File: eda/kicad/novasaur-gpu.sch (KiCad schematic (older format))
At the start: 24 parts, among them U1 74F86, U28 74F163, U29 74F163, U3 74F11, U30 74F541, U31 74F574, U32 74F574, U33 74F541, U34 74F574, U35 74F299, U36 74F574, U37 74F157

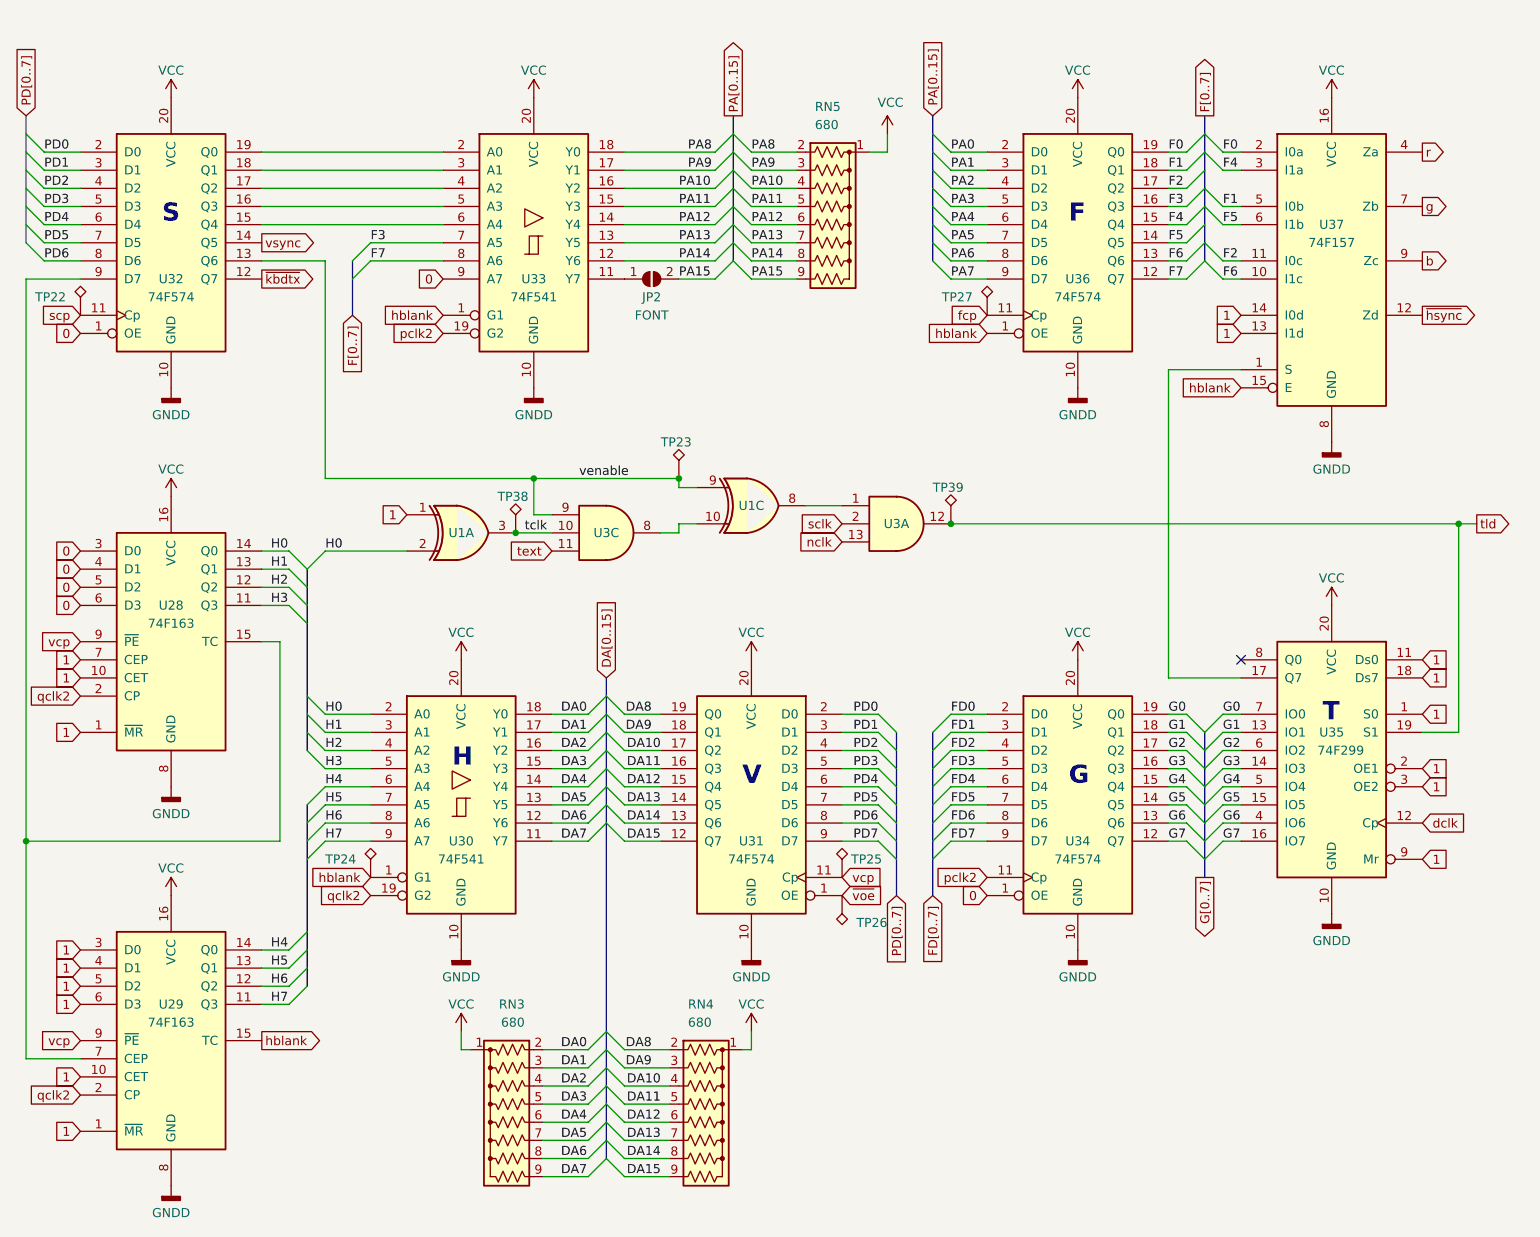
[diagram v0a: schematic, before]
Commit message: Rev. 10 with 5v PSU
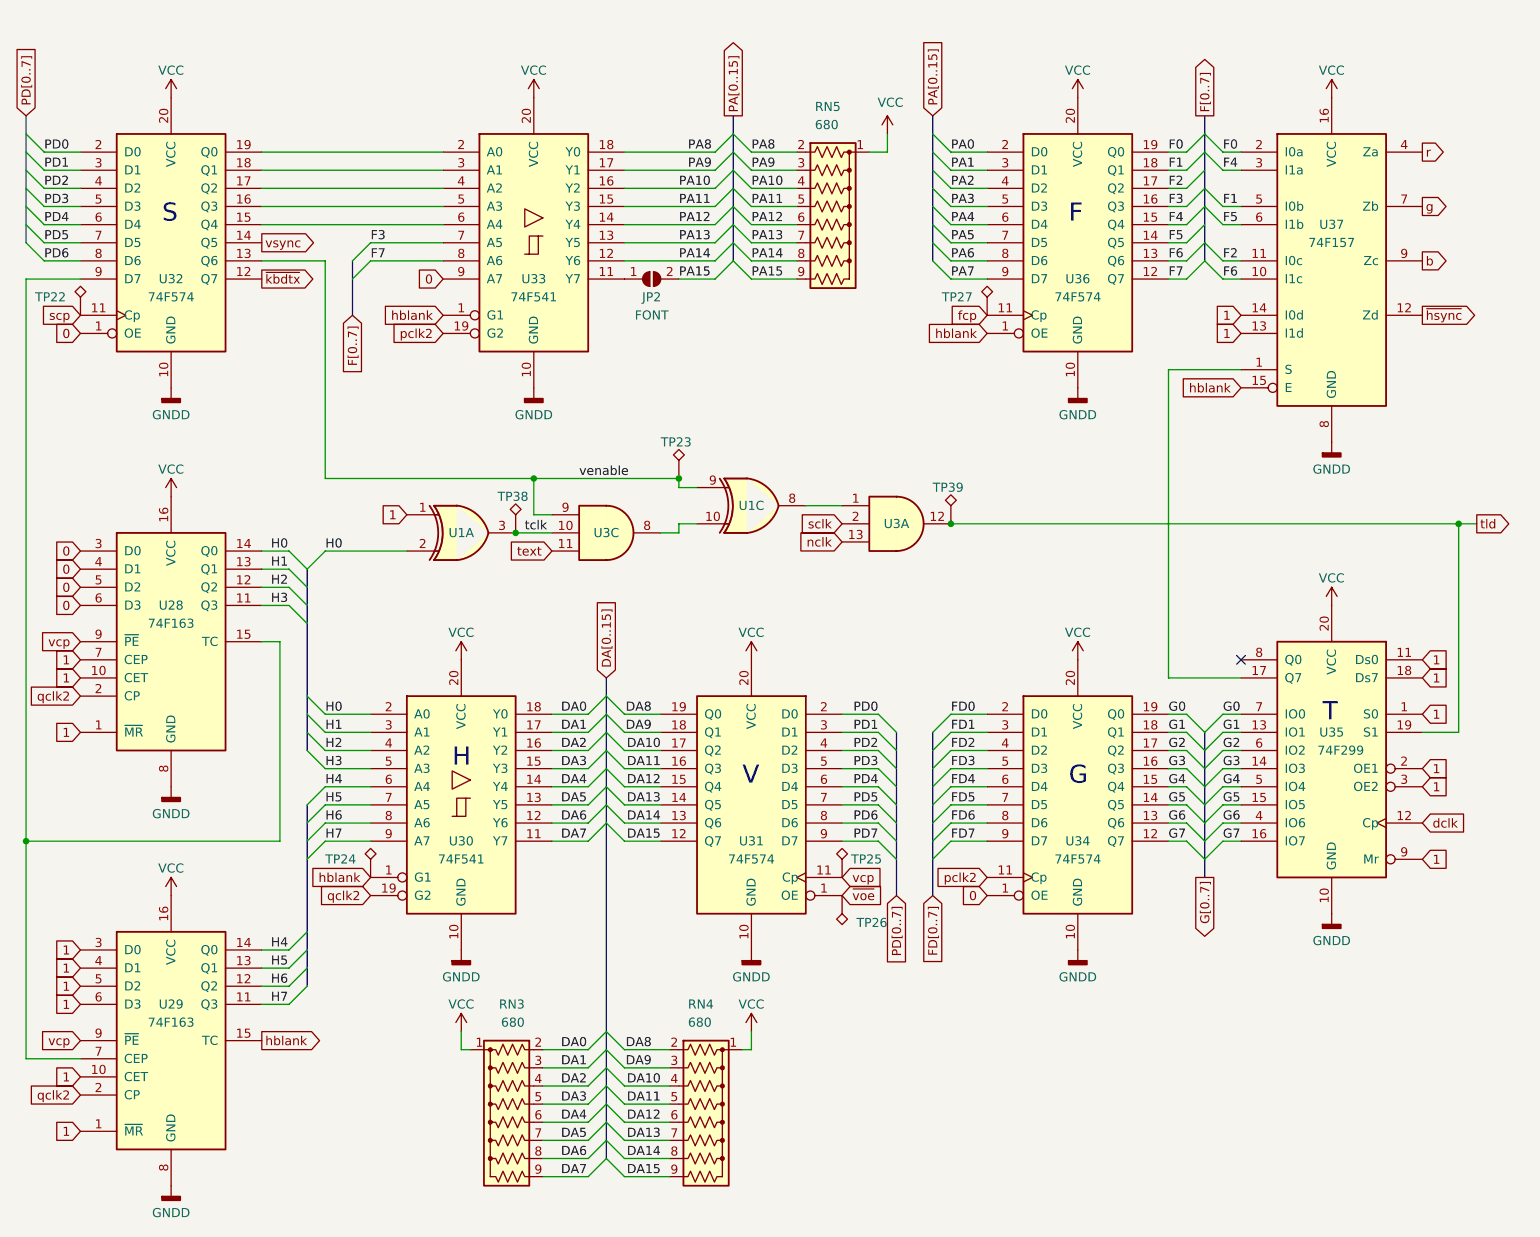
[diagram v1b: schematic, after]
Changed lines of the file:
@@
 Sheet 3 4
 Title "Graphics Processing Unit"
-Date "2021-08-01"
+Date "2021-09-02"
 Rev "1.10"
 Comp ""
@@
 Wire Wire Line
 	4200 3350 5000 3350
-Text Notes 3750 4950 0    100  ~ 20
+Text Notes 3750 4950 0    100  ~ 0
 H
-Text Notes 5350 5050 0    100  ~ 20
+Text Notes 5350 5050 0    100  ~ 0
 V
-Text Notes 7150 1950 0    100  ~ 20
+Text Notes 7150 1950 0    100  ~ 0
 F
-Text Notes 7150 5050 0    100  ~ 20
+Text Notes 7150 5050 0    100  ~ 0
 G
-Text Notes 2150 1950 0    100  ~ 20
+Text Notes 2150 1950 0    100  ~ 0
 S
-Text Notes 8550 4700 0    100  ~ 20
+Text Notes 8550 4700 0    100  ~ 0
 T
 Wire Bus Line
